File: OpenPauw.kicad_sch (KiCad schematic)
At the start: 10 parts, among them J1 Conn_01x01, J2 Conn_01x01, J3 Conn_01x01, J4 Conn_01x01, J5 Conn_01x04, U1 MAX328EPE+, U2 MAX328EPE+, U3 MAX328EPE+, U4 MAX328EPE+, U5 Adafruit-Feather-RP2040

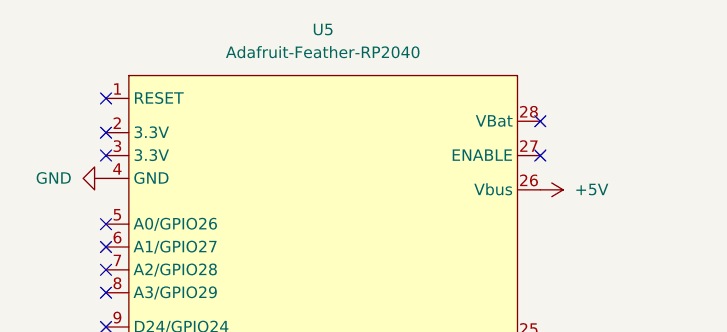
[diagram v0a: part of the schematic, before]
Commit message: New layout
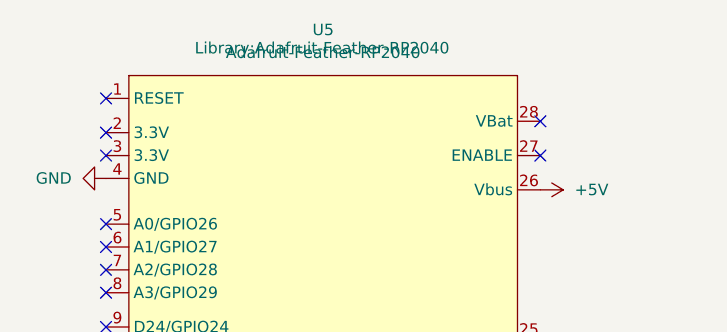
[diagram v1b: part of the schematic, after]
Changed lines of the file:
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@@
 					(size 1.27 1.27)
 				)
-				(hide yes)
 			)
 		)
